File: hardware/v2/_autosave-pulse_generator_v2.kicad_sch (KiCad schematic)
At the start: 27 parts, among them J1 Power, J2 Digital/PWM, J3 Analog, J4 Digital/PWM, J5 Conn_Coaxial, J6 Conn_Coaxial, SW1 SW_Push, U1 LM311, U2 74LS279

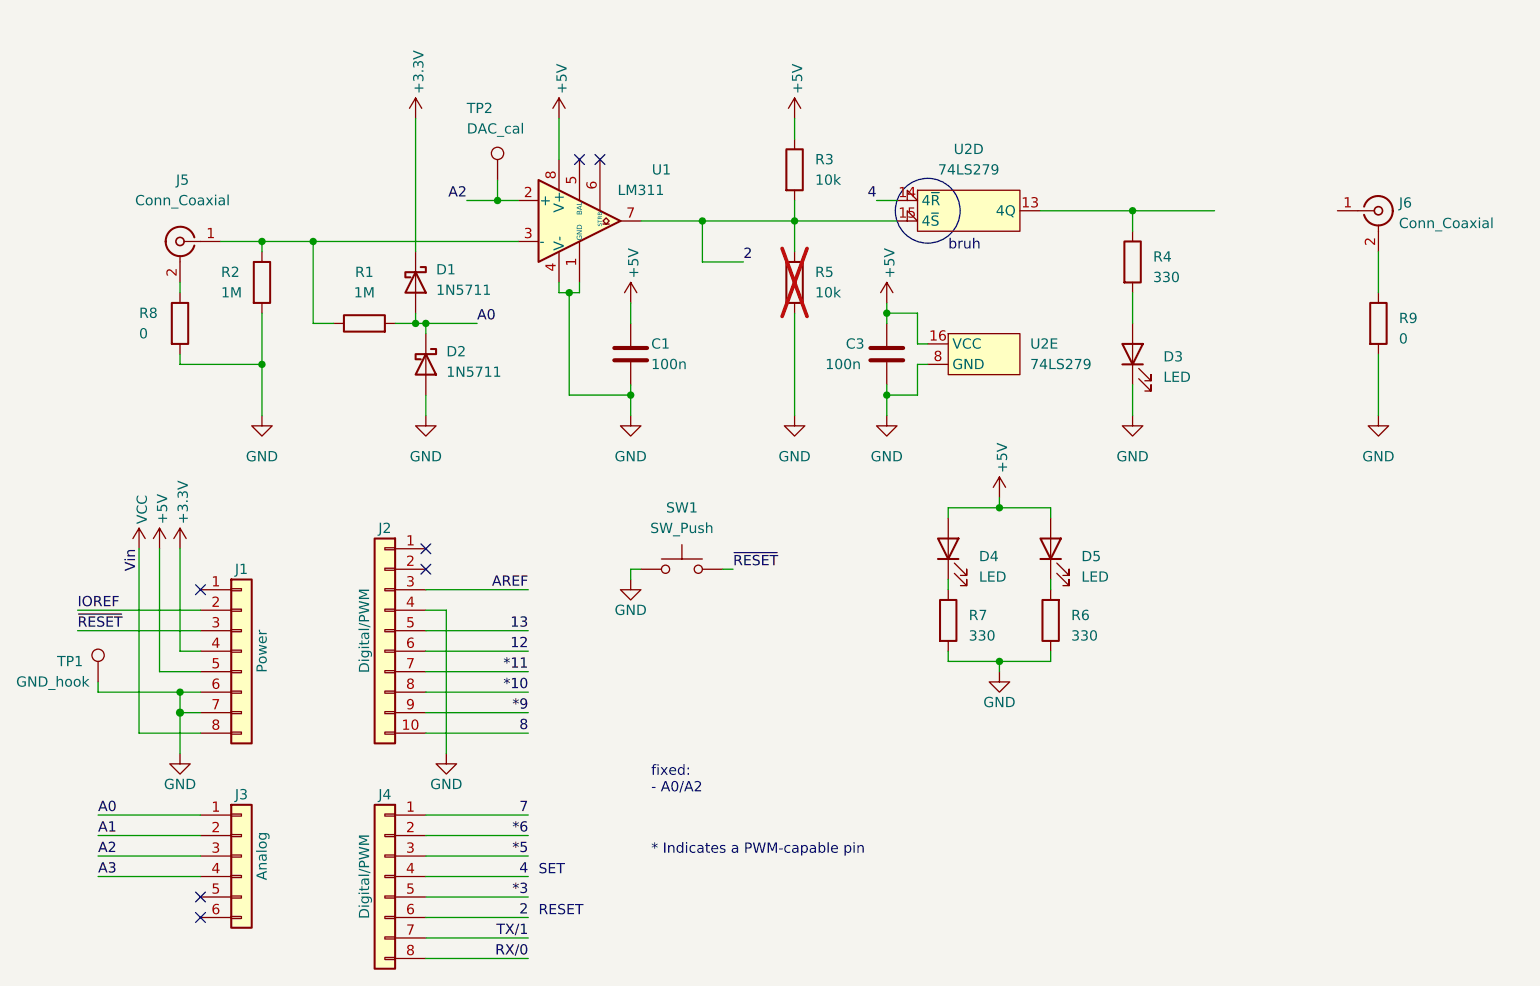
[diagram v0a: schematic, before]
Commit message: autosaves
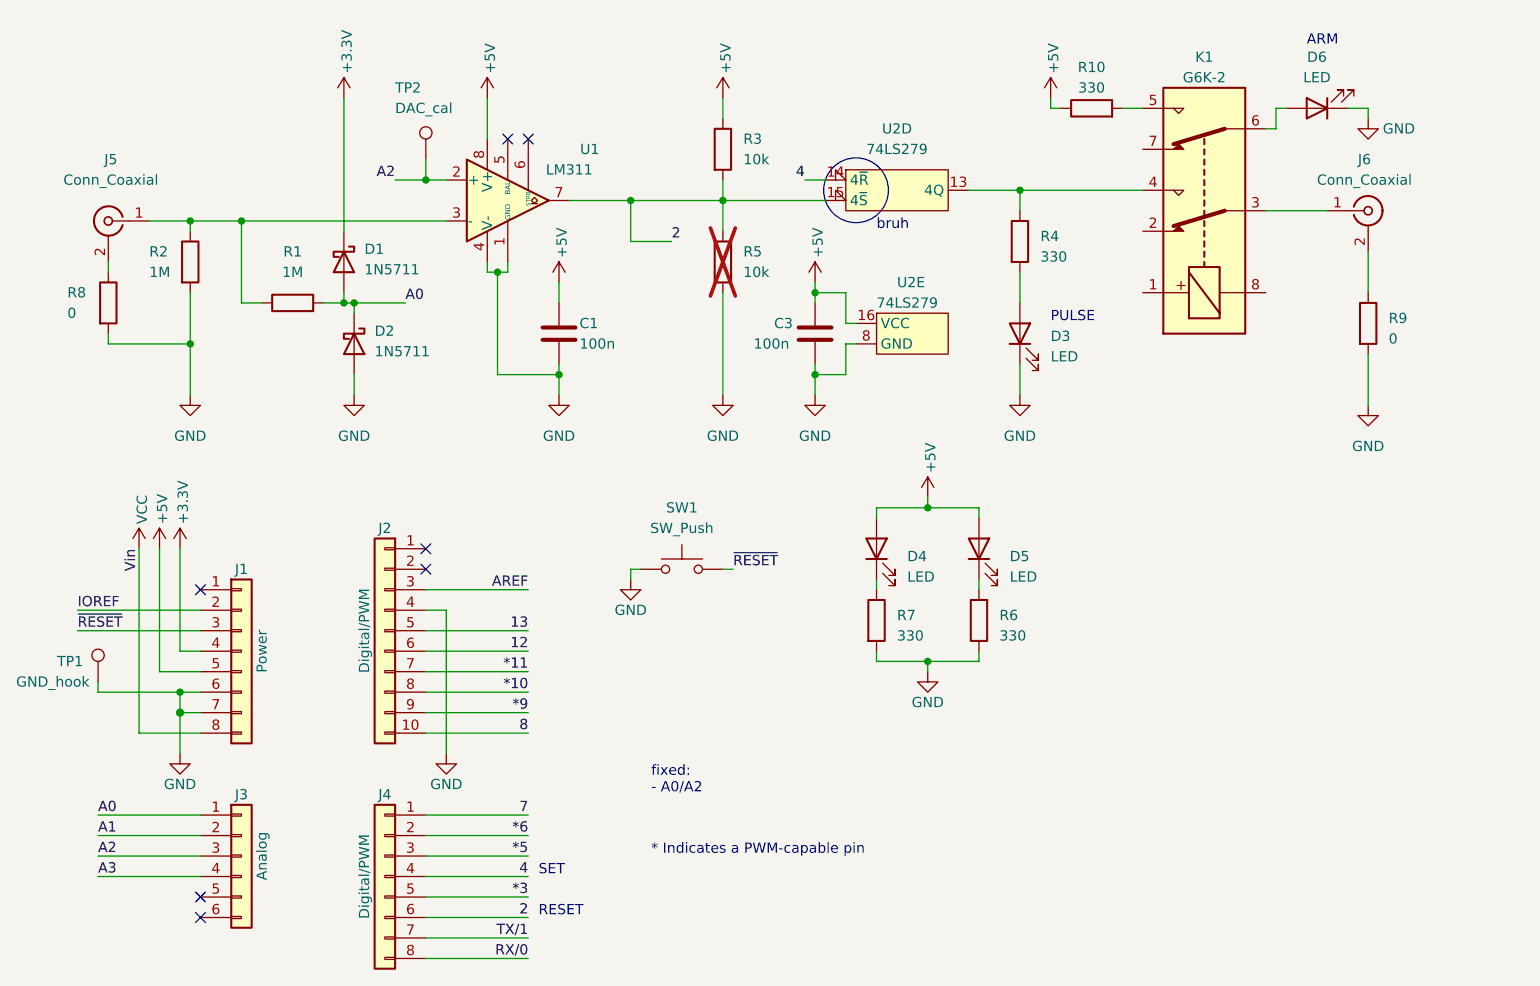
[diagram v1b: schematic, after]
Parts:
- added D6: LED, LED_THT:LED_D5.0mm, symbol Device:LED
- added K1: G6K-2, Relay_SMD:Relay_DPDT_Omron_G6K-2F-Y, symbol Relay:G6K-2
- added R10: 330, Resistor_SMD:R_0805_2012Metric_Pad1.20x1.40mm_HandSolder, symbol Device:R
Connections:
- net +5V: now also R10.1
- net GND: now also D6.1 (K)
- net at J6.1 (In): now also K1.3
- net at R4.1, U2.13 (4Q): now also K1.4
- new net: D6.2 (A), K1.6
- new net: K1.5, R10.2
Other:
- note added: "ARM"
- note added: "PULSE"
- moved on the sheet: C1, C3, D1, D2, D3, D4, D5, J5, J6, R1, R2, R3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
